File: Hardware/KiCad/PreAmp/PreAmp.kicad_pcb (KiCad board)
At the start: 2 copper layers, 26 parts, among them J1 XLR3, J2 Conn_01x05_Pin, U1 TLV2371DBV, U2 INA217AIDWR

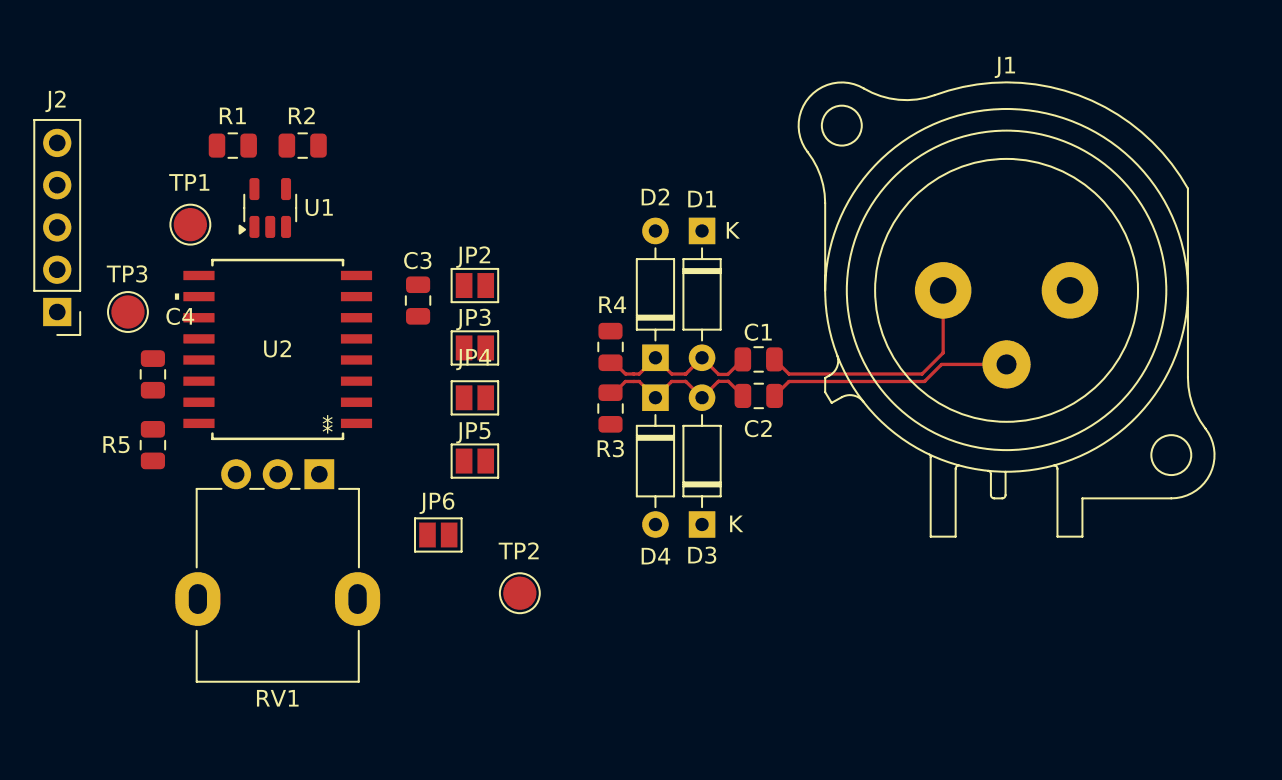
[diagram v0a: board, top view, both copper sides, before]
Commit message: Connected everything together
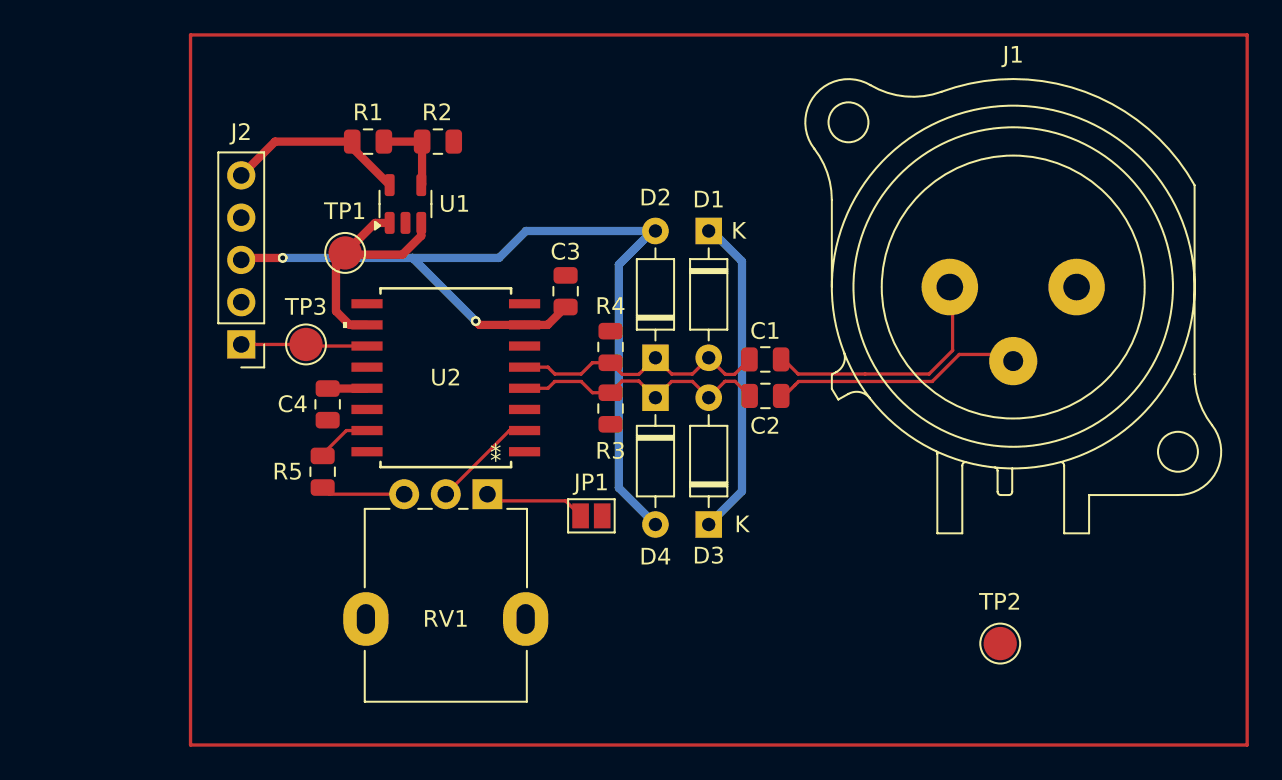
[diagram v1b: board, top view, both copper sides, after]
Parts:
- removed JP2, JP3, JP4, JP5: SolderJumper_2_Open, Jumper:SolderJumper-2_P1.3mm_Open_Pad1.0x1.5mm
- moved TP2 29.0 mm to (198.5, 87.4)
- moved J2 11.2 mm to (152.9, 69.4)
- moved TP3 10.9 mm to (156.8, 69.4)
- moved C4 10.7 mm to (158.1, 73.0)
- moved R5 10.3 mm to (157.8, 77.0)
- moved U2 10.2 mm to (165.2, 71.4)
- moved RV1 10.2 mm to (167.7, 78.4)
- moved TP1 9.46 mm to (159.2, 63.9)
- moved JP1 9.27 mm to (173.9, 79.7)
- moved C3 8.88 mm to (172.4, 66.2)
- moved R2 8.13 mm to (164.7, 57.2)
- moved R1 8.13 mm to (160.5, 57.2)
- moved U1 8.13 mm to (162.8, 61.0)
- moved J1 0.45 mm to (203.1, 66.0)
- moved C1 0.40 mm to (184.4, 70.3)
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- renumbered JP6 to JP1
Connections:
- net Input+ renamed /Input+
- net Input- renamed /Input-
- U2 pad 4: Net-(JP4-B) -> /In-
- U2 pad 5: Net-(JP2-B) -> /In+
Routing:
- net -6V: track 0.00 -> 56.5 mm, vias 0 -> 2
- net 6V: track 0.00 -> 32.8 mm
- net 1.6V: track 0.00 -> 15.2 mm
- net Out: track 0.00 -> 7.60 mm
- net Net-(U2-RG1): track 0.00 -> 6.32 mm
- net Net-(JP1-A): track 0.00 -> 6.14 mm
- net /In+: track 10.6 -> 16.6 mm
- net /In-: track 10.2 -> 16.3 mm
- net Net-(R5-Pad1): track 0.00 -> 5.07 mm
- net Net-(U1--): track 0.00 -> 4.93 mm
- net Net-(U2-RG2): track 0.00 -> 3.36 mm
